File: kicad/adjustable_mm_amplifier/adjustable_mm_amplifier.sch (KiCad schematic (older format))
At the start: 23 parts

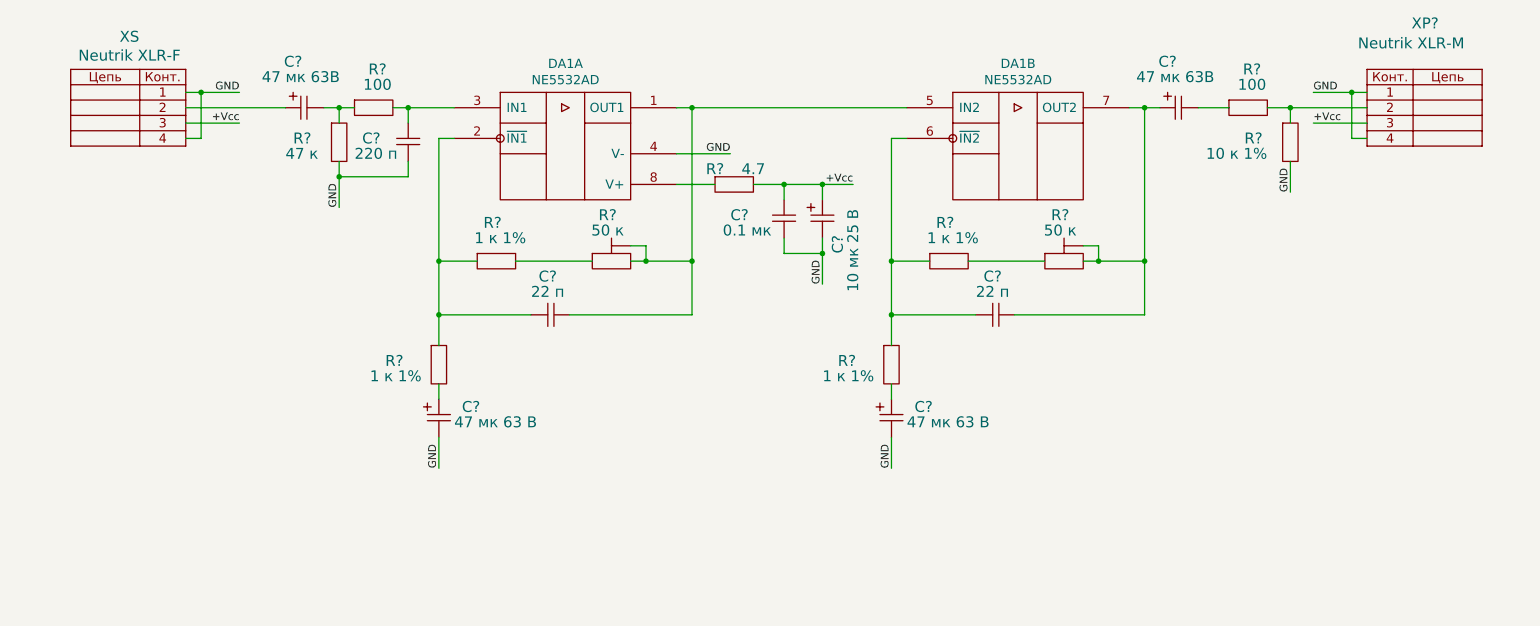
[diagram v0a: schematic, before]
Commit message: Закончил разрабатывать схему усилителя для микрофонов.
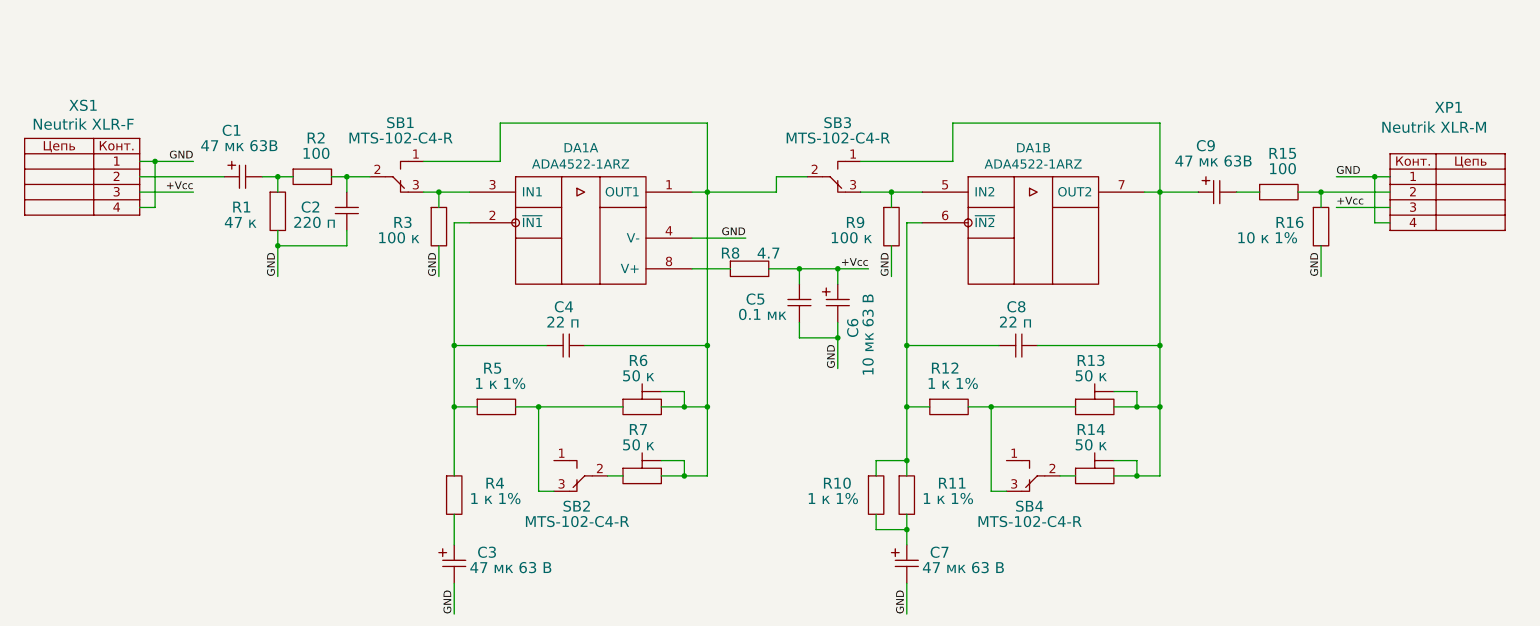
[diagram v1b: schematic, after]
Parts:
- removed C?: 47 мк 63 В, symbol LFcapitors:CAPITORS_ELECTROLYTIC
- removed C?: 22 п, symbol LFcapitors:CAPITORS
- removed R? (x3): 1 к 1%, symbol LFresistor:RESISTOR
- removed R?: 50 к, symbol LFresistor:RESISTOR_TRIMMING
- added C7: 47 мк 63 В, symbol LFcapitors:CAPITORS_ELECTROLYTIC
- added C8: 22 п, symbol LFcapitors:CAPITORS
- added R10, R11, R12, R4: 1 к 1%, symbol LFresistor:RESISTOR
- added R13, R14, R7: 50 к, symbol LFresistor:RESISTOR_TRIMMING
- added R3, R9: 100 к, symbol LFresistor:RESISTOR
- added SB1, SB2, SB3, SB4: MTS-102-C4-R, symbol LFbutton:MTS-102-C4-R
- C6: renamed from C?; value 10 мк 25 В -> 10 мк 63 В
- DA1: value NE5532AD -> ADA4522-1ARZ
- gave numbers to parts that had none: 14
- renumbered XS to XS1
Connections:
- net GND: now also C7.2, R3.2, R9.2
- net at C4.1, DA1.1 (OUT1), R6.2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: now also R7.2, R7.3, SB1.1, SB3.2; no longer DA1.5 (IN2)
- net at C4.2, DA1.2 (~IN1), R5.1: now also R4.1
- net at C2.1, R2.2: now also SB1.2; no longer DA1.3 (IN1)
- net at DA1.6 (~IN2): now also C8.2, R10.1, R11.1, R12.1
- net at C9.1, DA1.7 (OUT2): now also C8.1, R13.2, R13.3, R14.2, R14.3, SB3.1
- net at R5.2, R6.1: now also SB2.3
- net at C3.1: now also R4.2
- new net: DA1.3 (IN1), R3.1, SB1.3
- new net: DA1.5 (IN2), R9.1, SB3.3
- new net: R7.1, SB2.2
- new net: R12.2, R13.1, SB4.3
- new net: C7.1, R10.2, R11.2
- new net: R14.1, SB4.2
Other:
- moved on the sheet: C1, C2, C3, C4, C5, C6, C9, DA1A, DA1B, R1, R15, R16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
